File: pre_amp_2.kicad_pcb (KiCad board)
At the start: 2 copper layers, 61.3 x 49.9 mm, 48 parts, among them J1 IN, J11 SW2_3, J12 SW2_1, J13 SW2_4, J14 SW5_3, J15 VR5_1, J16 OUT, J2 Vin, J3 GND, J4 VR1_1, J5 VR2_1, J6 VR1_3, J7 VR1_2, J8 SW1, J9 SW2, U1 TL072, U2 ICL7660

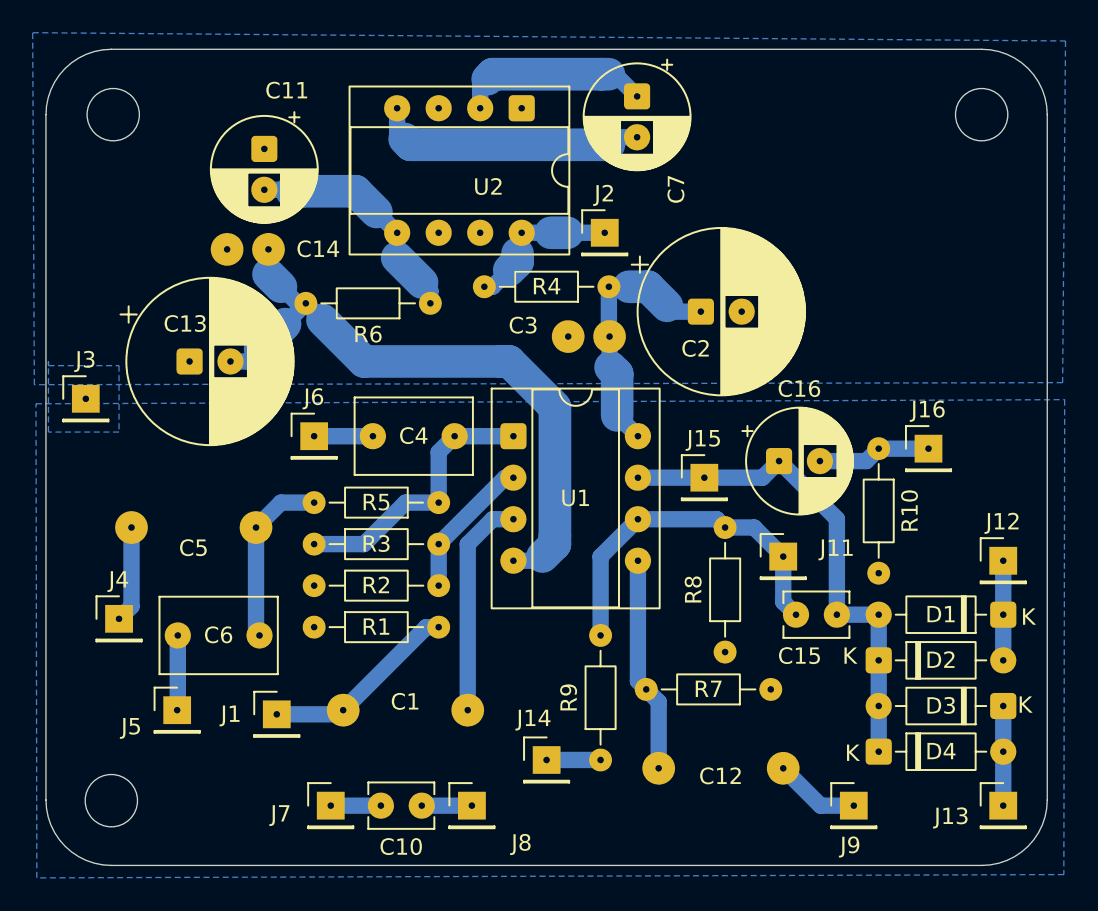
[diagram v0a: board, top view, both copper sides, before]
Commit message: 配置修正
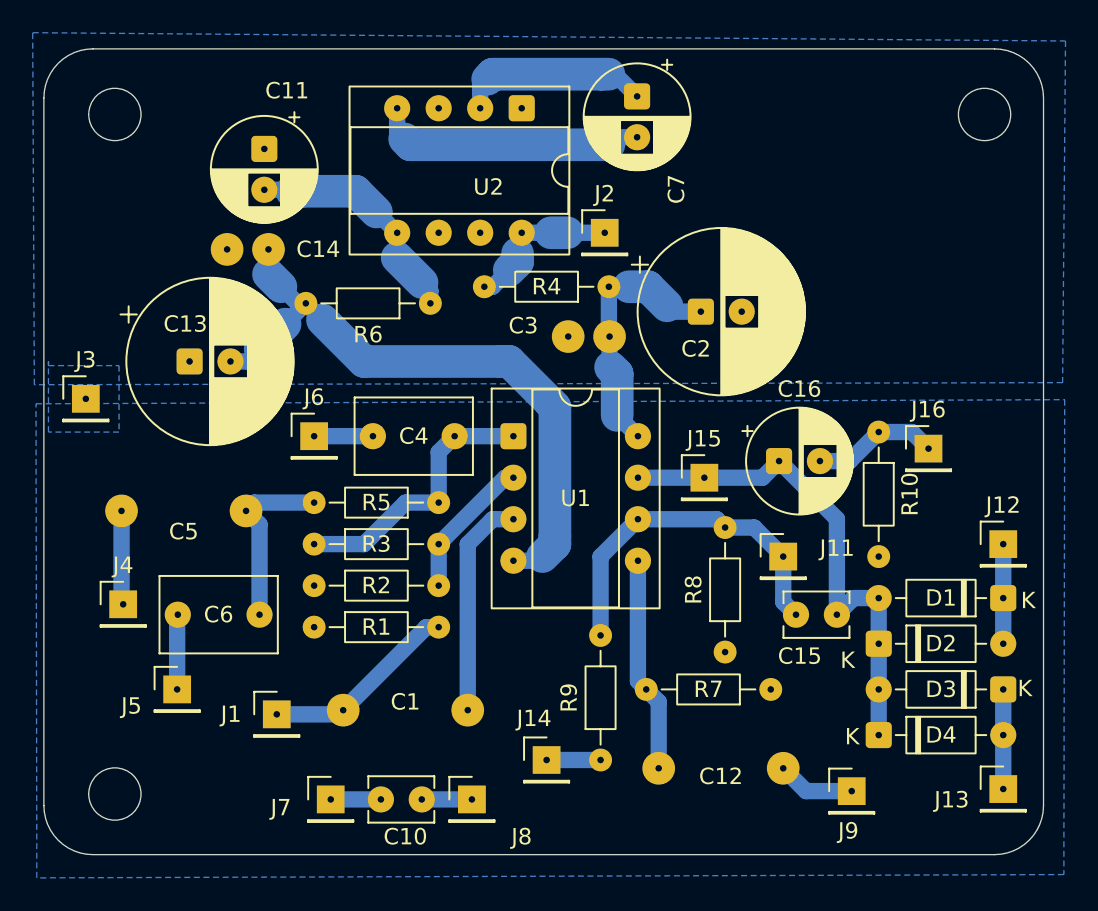
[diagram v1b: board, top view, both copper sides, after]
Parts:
- moved C6 1.27 mm to (127.5, 107.2)
- moved J5 1.27 mm to (122.4, 111.8)
- moved C5 1.18 mm to (122.8, 100.8)
- moved D1 1.02 mm to (173.0, 106.2)
- moved D2 1.02 mm to (165.4, 109.0)
- moved J13 1.02 mm to (173.0, 117.9)
- moved R10 1.02 mm to (165.4, 96.0)
- moved D3 1.02 mm to (173.0, 111.8)
- moved D4 1.02 mm to (165.4, 114.6)
- moved J12 1.02 mm to (173.0, 102.9)
- moved J4 0.92 mm to (119.1, 106.6)
- moved J9 0.90 mm to (163.7, 118.0)
- moved H3 0.46 mm to (118.6, 118.2)
- moved C10 0.38 mm to (134.9, 118.5)
- moved J7 0.38 mm to (131.8, 118.5)
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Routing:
- net Net-(J16-Pin_1): track 6.96 -> 7.80 mm
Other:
- board size 61.3 x 49.9 mm -> 61.2 x 49.3 mm
